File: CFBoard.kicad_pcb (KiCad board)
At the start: 2 copper layers, 80 x 60 mm, 24 parts, among them SW1 Slide Switch, U1 STM32 Blue Pill, U2 Wemos D1 Mini, U3 GY-6500, U4 BMP180_5pin

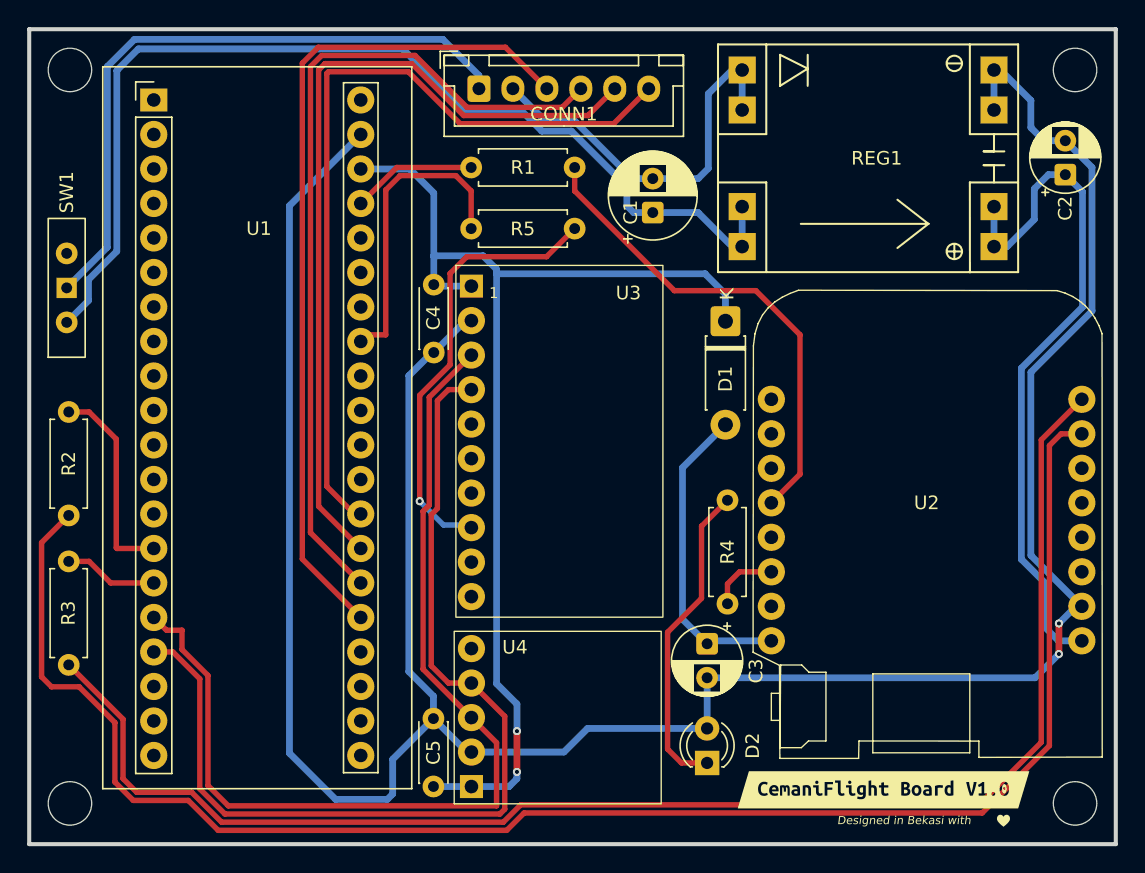
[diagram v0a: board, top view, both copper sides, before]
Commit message: feat: update design
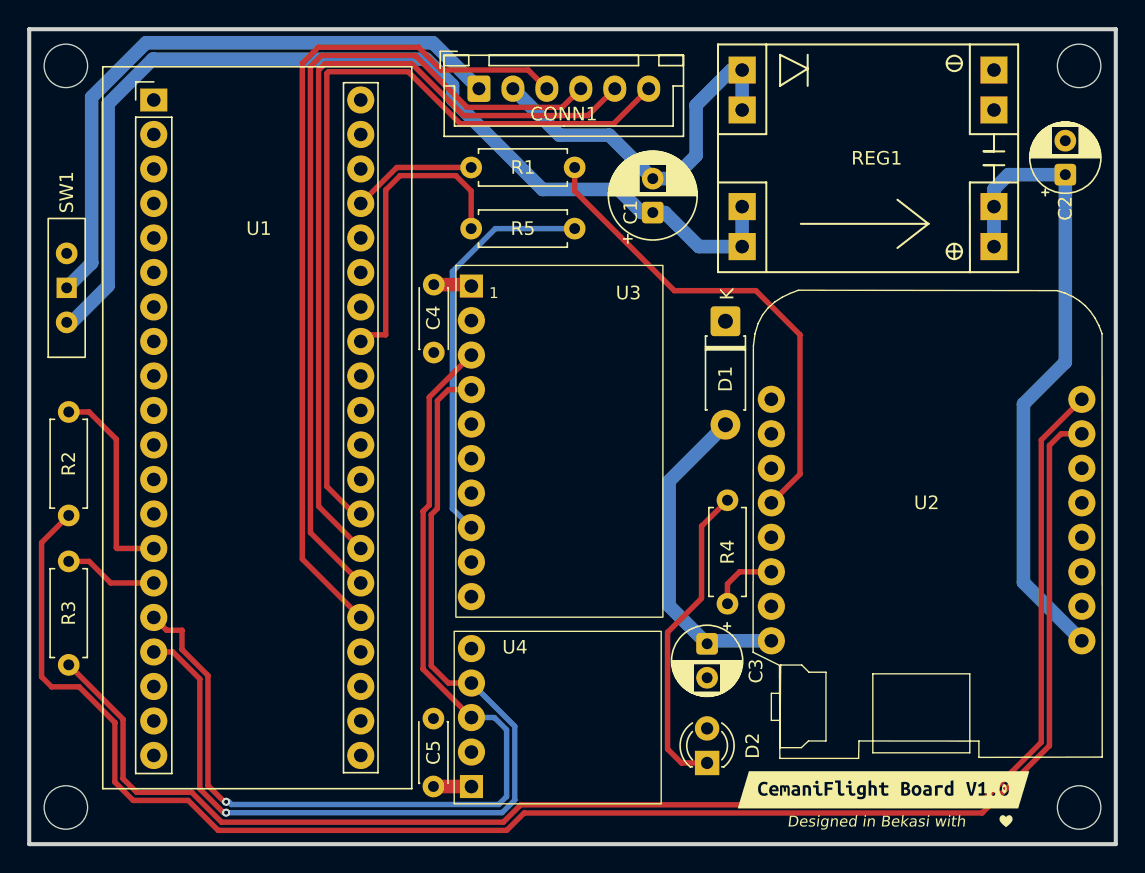
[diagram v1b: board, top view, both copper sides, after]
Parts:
- removed the REF** at (182.5, 132.0)
- removed the REF** at (108.5, 132.0)
- removed the REF** at (182.5, 78.0)
- removed the REF** at (108.5, 78.0)
- added REF**: MountingHole_3.2mm_M3_DIN965, MountingHole:MountingHole_3.2mm_M3_DIN965, F.Cu at (108.2, 132.3)
- added REF**: MountingHole_3.2mm_M3_DIN965, MountingHole:MountingHole_3.2mm_M3_DIN965, F.Cu at (182.8, 77.7)
- added REF**: MountingHole_3.2mm_M3_DIN965, MountingHole:MountingHole_3.2mm_M3_DIN965, F.Cu at (108.2, 77.7)
- added REF**: MountingHole_3.2mm_M3_DIN965, MountingHole:MountingHole_3.2mm_M3_DIN965, F.Cu at (182.8, 132.3)
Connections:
- net Net-(D1-K) renamed DIODPWR
- net Net-(D2-A) renamed GNDREG
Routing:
- net GNDREG: track 200.9 -> 0.00 mm, vias 2 -> 0
- net DIODPWR: track 84.5 -> 5.45 mm, vias 2 -> 0
- net Net-(REG1-VOUT+): track 51.3 -> 47.3 mm
- net Net-(U3-INT): track 32.6 -> 29.7 mm, vias 1 -> 0
- net Net-(U1-PB8): track 73.5 -> 75.0 mm, vias 0 -> 1
- net Net-(CONN1-VIN): track 47.8 -> 46.4 mm
- net Net-(REG1-VIN+): track 75.8 -> 74.9 mm
- net Net-(D1-A): track 22.7 -> 23.5 mm
- net Net-(U1-PB9): track 72.0 -> 72.6 mm, vias 0 -> 1
- added copper zone on F.Cu, net DIODPWR
- added copper zone on B.Cu, net GNDREG
